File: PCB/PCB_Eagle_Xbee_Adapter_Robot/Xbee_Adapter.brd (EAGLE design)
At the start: 55.7 x 55.2 mm, 34 parts, among them IC1 LD117AS33TR, U1 CY8C4247AZI-M485

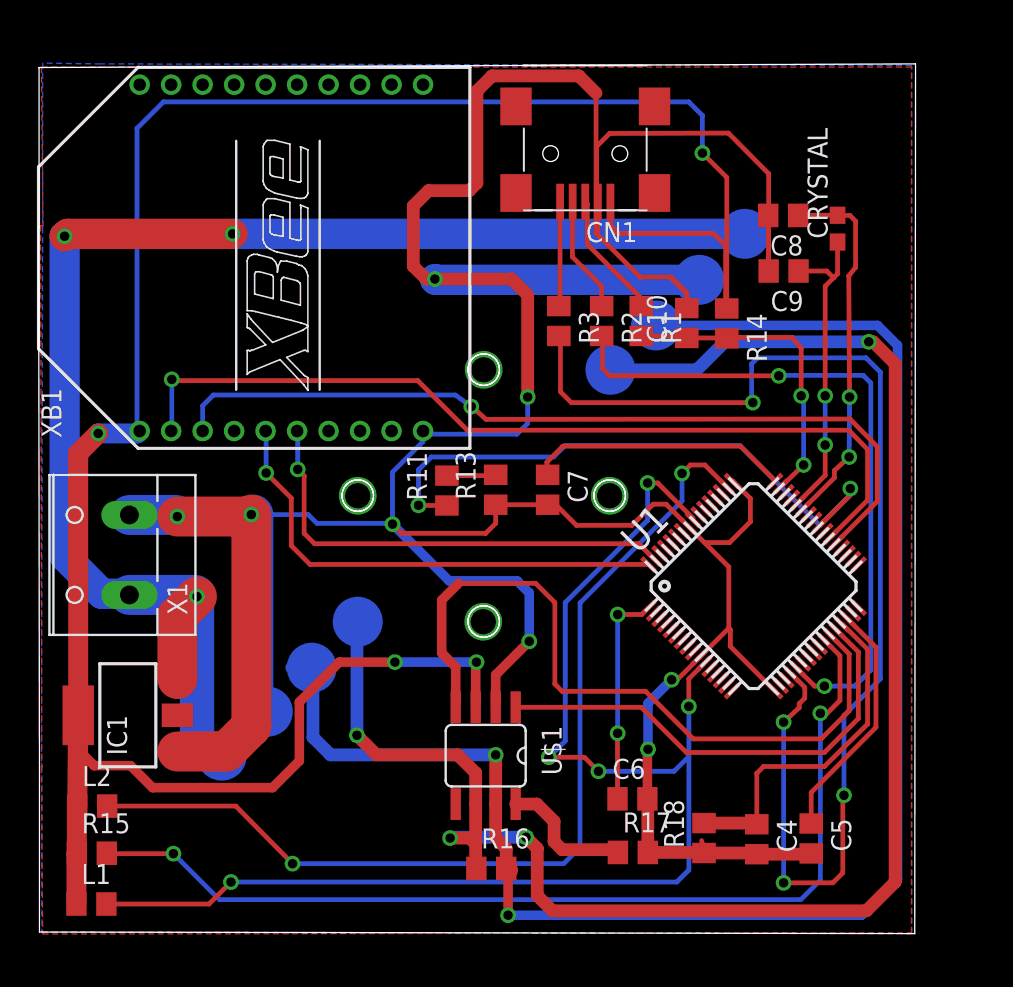
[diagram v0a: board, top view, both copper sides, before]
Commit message: ULTIMA EDICION
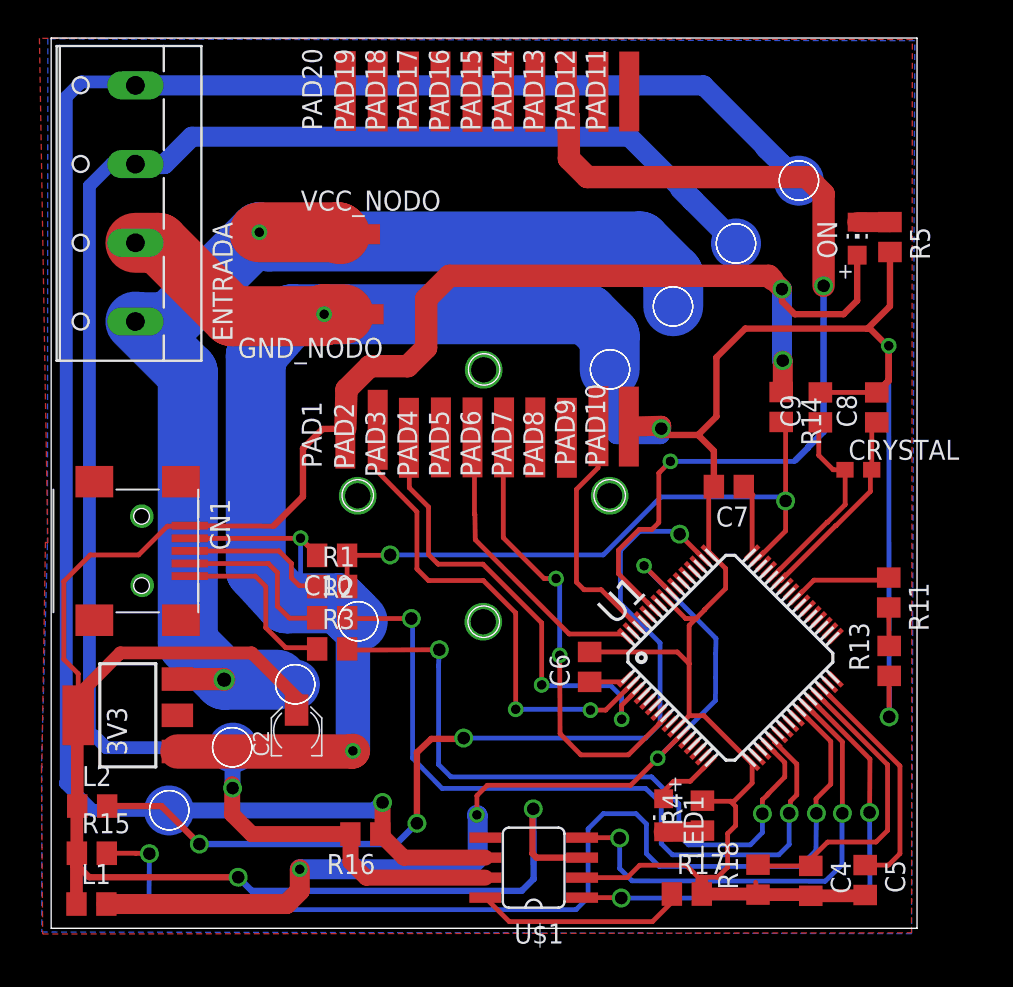
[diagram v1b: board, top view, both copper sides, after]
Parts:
- removed X1: (no value), con-wago-508:W237-132
- removed XB1: XBEE, xbee:XBEE
- added C2: (no value), rcl:PANASONIC_A
- added ENTRADA: (no value), con-wago-500:W237-4
- added GND_NODO, PAD1, PAD10, PAD11, PAD12, PAD13, PAD14, PAD15, PAD16, PAD17, PAD18, PAD19, PAD2, PAD20, PAD3, PAD4, PAD5, PAD6, PAD7, PAD8, PAD9, VCC_NODO: (no value), wirepad:SMD2,54-5,08
- added LED1, ON: (no value), adafruit:CHIP-LED0805
- added R4: (no value), rcl:R0805
- added R5: 1K, rcl:R0805
- moved CN1 39.2 mm to (124.6, 82.9), turned to 270 degrees
- moved R11 28.8 mm to (173.1, 80.2), turned to 270 degrees
- moved R13 27.3 mm to (173.1, 75.9)
- moved C10 26.9 mm to (137.7, 82.6), turned to 180 degrees
- moved R1 25.9 mm to (137.7, 80.6), turned to 0 degrees
- moved R2 25.5 mm to (137.7, 78.6), turned to 0 degrees
- moved R3 25.3 mm to (137.7, 76.6), turned to 0 degrees
- moved CANL_1_C2 17.0 mm to (167.3, 106.4)
- moved CANL_1_C1 17.0 mm to (127.3, 66.4)
- moved CRYSTAL 15.4 mm to (171.1, 88.0), turned to 0 degrees
- moved C8 13.6 mm to (172.3, 92.0), turned to 90 degrees
- moved C7 11.5 mm to (162.9, 86.9), turned to 180 degrees
- moved C9 8.97 mm to (168.7, 92.0), turned to 90 degrees
- moved C6 8.81 mm to (154.1, 75.5), turned to 90 degrees
- moved R16 8.29 mm to (139.8, 64.9), turned to 180 degrees
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- renumbered IC1 to 3V3
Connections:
- new net N$10: ON.C, R5.1
- new net N$5: LED1.A, U1.16
- new net N$6: LED1.C, R4.1
- new net SLEEP_CTRL: PAD9.1, U1.62
- new net SLEEP_XBEE: PAD13.1, U1.59
- net 3V3: now also C2.+, ON.A, PAD1.1; no longer XB1.1
- net CANH: now also ENTRADA.3
- net CANL: now also ENTRADA.4
- net GND: now also C2.-, ENTRADA.2, GND_NODO.1, PAD10.1, R4.2, R5.2; no longer X1.2, XB1.10
- net RESET_XBEE: now also PAD5.1; no longer XB1.5
- net RX_STRENGTH: now also PAD6.1, U1.8; no longer U1.63, XB1.6
- net UART_RX: now also PAD3.1, U1.3; no longer U1.37, XB1.3
- net UART_TX: now also PAD2.1, U1.2; no longer U1.38, XB1.2
- net VCC_9-12V: now also ENTRADA.1, VCC_NODO.1; no longer X1.1
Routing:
- net SLEEP_XBEE: track 0.00 -> 59.1 mm, vias 0 -> 2
- net SWDIO: track 78.3 -> 43.8 mm, vias 4 -> 2
- net P0_1: track 39.0 -> 6.36 mm, vias 2 -> 0
- net UART_TX: track 55.8 -> 31.5 mm, vias 1 -> 2
- net UART_RX: track 53.2 -> 29.9 mm, vias 1 -> 2
- net VDDA: track 85.0 -> 62.1 mm, vias 5 -> 4
- net XRES: track 20.0 -> 41.1 mm
- net CANL: track 108.7 -> 126.6 mm, vias 4 -> 1
- net CAN_RX: track 46.6 -> 30.1 mm, vias 0 -> 2
- net SLEEP_CTRL: track 0.00 -> 15.4 mm
- net RESET_XBEE: track 31.1 -> 18.6 mm, vias 1 -> 0
- net VCCD: track 16.7 -> 4.41 mm
- net SAR_BY: track 13.8 -> 2.32 mm, vias 2 -> 0
- net P0_4: track 23.5 -> 12.6 mm, vias 2 -> 0
- net CANH: track 103.8 -> 114.0 mm, vias 2 -> 1
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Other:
- board size 55.7 x 55.2 mm -> 55 x 56.5 mm
